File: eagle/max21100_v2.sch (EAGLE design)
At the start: 11 parts

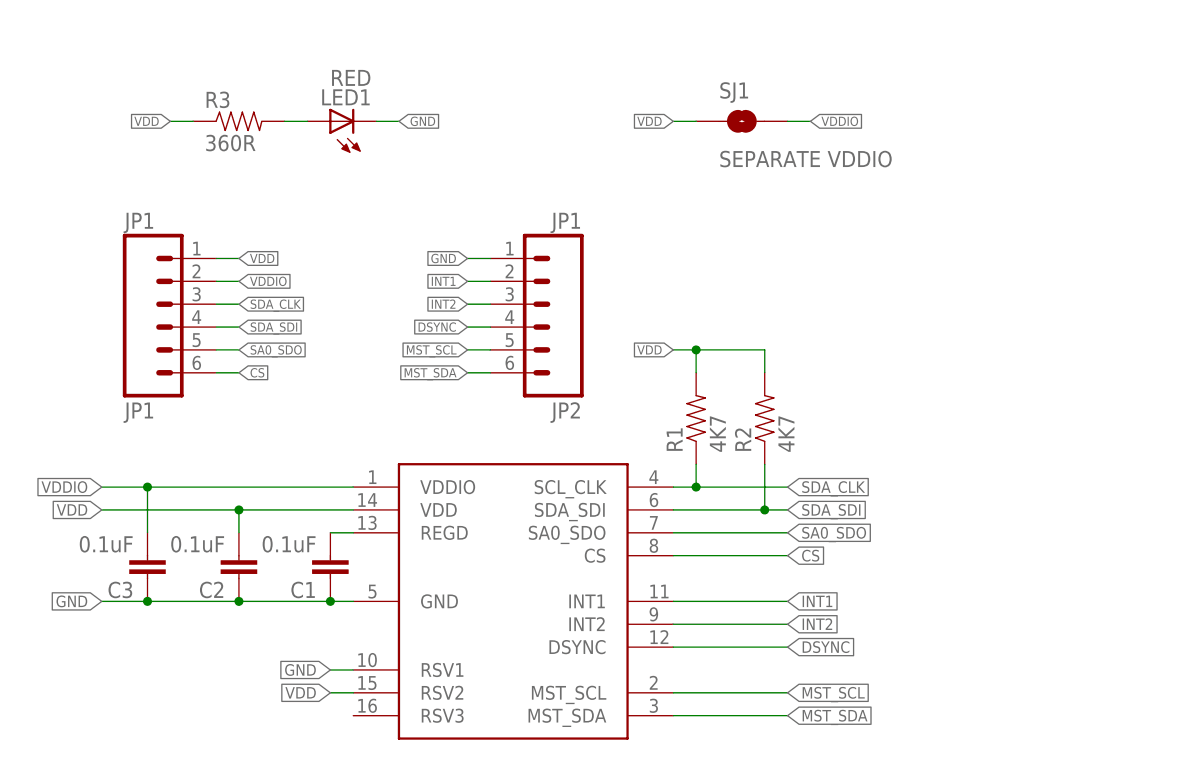
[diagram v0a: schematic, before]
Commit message: Improved V2
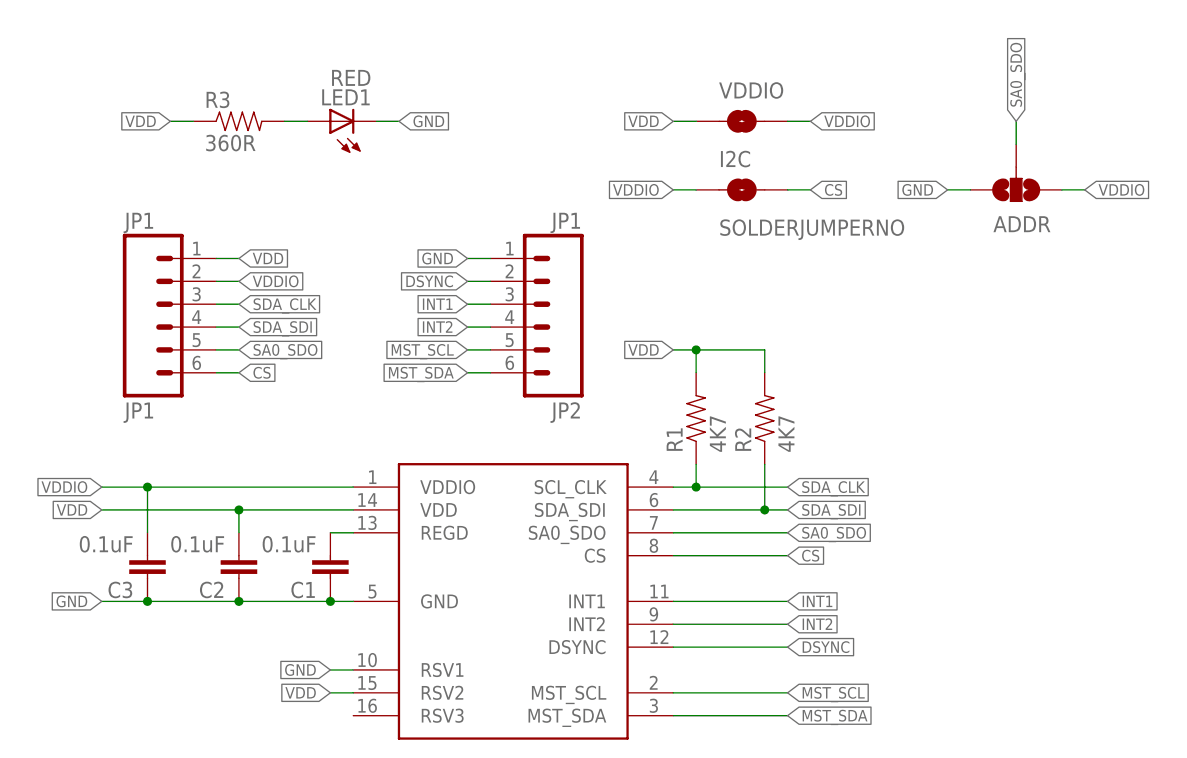
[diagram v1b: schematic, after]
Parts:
- added ADDR: (no value), max21100:SOLDERJUMPER_2WAYS
- added I2C: SOLDERJUMPERNO, max21100:SOLDERJUMPERNO
- VDDIO: value SEPARATE VDDIO -> SOLDERJUMPERTRACE
- renumbered SJ1 to VDDIO
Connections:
- net CS: now also I2C.2
- net DSYNC: now also JP2.2; no longer JP2.4
- net GND: now also ADDR.1
- net INT1: now also JP2.3; no longer JP2.2
- net INT2: now also JP2.4; no longer JP2.3
- net SA0_SDO: now also ADDR.2
- net VDDIO: now also ADDR.3, I2C.1
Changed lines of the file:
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@@
 <part name="R3" library="SparkFun-Passives" deviceset="RESISTOR" device="0603-RES" value="360R"/>
 <part name="LED1" library="breakouts" deviceset="LED" device="CHIP-LED0603" value="RED"/>
-<part name="SJ1" library="max21100" deviceset="SOLDERJUMPER" device="TRACE" value="SEPARATE VDDIO"/>
+<part name="VDDIO" library="max21100" deviceset="SOLDERJUMPER" device="TRACE" value=""/>
+<part name="I2C" library="max21100" deviceset="SOLDERJUMPER" device="NO" value="SOLDERJUMPERNO"/>
+<part name="ADDR" library="max21100" deviceset="SOLDERJUMPER_2WAY" device="S"/>
 </parts>
 <sheets>
@@
 <instance part="R3" gate="G$1" x="40.64" y="99.06"/>
 <instance part="LED1" gate="G$1" x="50.8" y="99.06" rot="R90"/>
-<instance part="SJ1" gate="1" x="96.52" y="99.06"/>
+<instance part="VDDIO" gate="1" x="96.52" y="99.06"/>
+<instance part="I2C" gate="1" x="96.52" y="91.44"/>
+<instance part="ADDR" gate="G$1" x="127" y="91.44" smashed="yes" rot="MR270">
+<attribute name="NAME" x="124.46" y="88.519" size="1.778" layer="95" rot="MR180"/>
+<attribute name="VALUE" x="128.905" y="88.9" size="1.778" layer="96" rot="MR270"/>
+</instance>
 </instances>
 <busses>
@@
 <segment>
 <wire x1="55.88" y1="99.06" x2="58.42" y2="99.06" width="0.1524" layer="91"/>
-<label x="58.42" y="99.06" size="1.016" layer="95" xref="yes"/>
+<label x="58.42" y="99.06" size="1.27" layer="95" xref="yes"/>
 <pinref part="LED1" gate="G$1" pin="C"/>
 </segment>
@@
 <pinref part="JP2" gate="G$1" pin="1"/>
 <wire x1="68.58" y1="83.82" x2="66.04" y2="83.82" width="0.1524" layer="91"/>
-<label x="66.04" y="83.82" size="1.016" layer="95" rot="R180" xref="yes"/>
+<label x="66.04" y="83.82" size="1.27" layer="95" rot="R180" xref="yes"/>
+</segment>
+<segment>
+<pinref part="ADDR" gate="G$1" pin="1"/>
+<wire x1="121.92" y1="91.44" x2="119.38" y2="91.44" width="0.1524" layer="91"/>
+<label x="119.38" y="91.44" size="1.27" layer="95" rot="R180" xref="yes"/>
 </segment>
 </net>
@@
 <wire x1="91.44" y1="73.66" x2="88.9" y2="73.66" width="0.1524" layer="91"/>
 <junction x="91.44" y="73.66"/>
-<label x="88.9" y="73.66" size="1.016" layer="95" rot="R180" xref="yes"/>
+<label x="88.9" y="73.66" size="1.27" layer="95" rot="R180" xref="yes"/>
 </segment>
 <segment>
 <wire x1="33.02" y1="99.06" x2="35.56" y2="99.06" width="0.1524" layer="91"/>
-<label x="33.02" y="99.06" size="1.016" layer="95" rot="R180" xref="yes"/>
+<label x="33.02" y="99.06" size="1.27" layer="95" rot="R180" xref="yes"/>
 <pinref part="R3" gate="G$1" pin="1"/>
 </segment>
@@
 <pinref part="JP1" gate="G$1" pin="1"/>
 <wire x1="38.1" y1="83.82" x2="40.64" y2="83.82" width="0.1524" layer="91"/>
-<label x="40.64" y="83.82" size="1.016" layer="95" xref="yes"/>
-</segment>
-<segment>
-<pinref part="SJ1" gate="1" pin="1"/>
+<label x="40.64" y="83.82" size="1.27" layer="95" xref="yes"/>
+</segment>
+<segment>
+<pinref part="VDDIO" gate="1" pin="1"/>
 <wire x1="91.44" y1="99.06" x2="88.9" y2="99.06" width="0.1524" layer="91"/>
-<label x="88.9" y="99.06" size="1.016" layer="95" rot="R180" xref="yes"/>
+<label x="88.9" y="99.06" size="1.27" layer="95" rot="R180" xref="yes"/>
 </segment>
 </net>
@@
 <pinref part="JP1" gate="G$1" pin="2"/>
 <wire x1="38.1" y1="81.28" x2="40.64" y2="81.28" width="0.1524" layer="91"/>
-<label x="40.64" y="81.28" size="1.016" layer="95" xref="yes"/>
-</segment>
-<segment>
-<pinref part="SJ1" gate="1" pin="2"/>
+<label x="40.64" y="81.28" size="1.27" layer="95" xref="yes"/>
+</segment>
+<segment>
+<pinref part="VDDIO" gate="1" pin="2"/>
 <wire x1="101.6" y1="99.06" x2="104.14" y2="99.06" width="0.1524" layer="91"/>
-<label x="104.14" y="99.06" size="1.016" layer="95" xref="yes"/>
+<label x="104.14" y="99.06" size="1.27" layer="95" xref="yes"/>
+</segment>
+<segment>
+<pinref part="I2C" gate="1" pin="1"/>
+<wire x1="91.44" y1="91.44" x2="88.9" y2="91.44" width="0.1524" layer="91"/>
+<label x="88.9" y="91.44" size="1.27" layer="95" rot="R180" xref="yes"/>
+</segment>
+<segment>
+<pinref part="ADDR" gate="G$1" pin="3"/>
+<wire x1="132.08" y1="91.44" x2="134.62" y2="91.44" width="0.1524" layer="91"/>
+<label x="134.62" y="91.44" size="1.27" layer="95" xref="yes"/>
 </segment>
 </net>
@@
 </segment>
 <segment>
-<pinref part="JP2" gate="G$1" pin="4"/>
-<wire x1="68.58" y1="76.2" x2="66.04" y2="76.2" width="0.1524" layer="91"/>
-<label x="66.04" y="76.2" size="1.016" layer="95" rot="R180" xref="yes"/>
+<pinref part="JP2" gate="G$1" pin="2"/>
+<wire x1="68.58" y1="81.28" x2="66.04" y2="81.28" width="0.1524" layer="91"/>
+<label x="66.04" y="81.28" size="1.27" layer="95" rot="R180" xref="yes"/>
 </segment>
 </net>
@@
 </segment>
 <segment>
-<pinref part="JP2" gate="G$1" pin="3"/>
-<wire x1="68.58" y1="78.74" x2="66.04" y2="78.74" width="0.1524" layer="91"/>
-<label x="66.04" y="78.74" size="1.016" layer="95" rot="R180" xref="yes"/>
+<pinref part="JP2" gate="G$1" pin="4"/>
+<wire x1="68.58" y1="76.2" x2="66.04" y2="76.2" width="0.1524" layer="91"/>
+<label x="66.04" y="76.2" size="1.27" layer="95" rot="R180" xref="yes"/>
 </segment>
 </net>
@@
 </segment>
 <segment>
-<pinref part="JP2" gate="G$1" pin="2"/>
-<wire x1="68.58" y1="81.28" x2="66.04" y2="81.28" width="0.1524" layer="91"/>
-<label x="66.04" y="81.28" size="1.016" layer="95" rot="R180" xref="yes"/>
+<pinref part="JP2" gate="G$1" pin="3"/>
+<wire x1="68.58" y1="78.74" x2="66.04" y2="78.74" width="0.1524" layer="91"/>
+<label x="66.04" y="78.74" size="1.27" layer="95" rot="R180" xref="yes"/>
 </segment>
 </net>
@@
 <pinref part="JP2" gate="G$1" pin="6"/>
 <wire x1="68.58" y1="71.12" x2="66.04" y2="71.12" width="0.1524" layer="91"/>
-<label x="66.04" y="71.12" size="1.016" layer="95" rot="R180" xref="yes"/>
+<label x="66.04" y="71.12" size="1.27" layer="95" rot="R180" xref="yes"/>
 </segment>
 </net>
@@
 <pinref part="JP2" gate="G$1" pin="5"/>
 <wire x1="68.58" y1="73.66" x2="66.04" y2="73.66" width="0.1524" layer="91"/>
-<label x="66.04" y="73.66" size="1.016" layer="95" rot="R180" xref="yes"/>
+<label x="66.04" y="73.66" size="1.27" layer="95" rot="R180" xref="yes"/>
 </segment>
 </net>
@@
 <pinref part="JP1" gate="G$1" pin="6"/>
 <wire x1="38.1" y1="71.12" x2="40.64" y2="71.12" width="0.1524" layer="91"/>
-<label x="40.64" y="71.12" size="1.016" layer="95" xref="yes"/>
+<label x="40.64" y="71.12" size="1.27" layer="95" xref="yes"/>
+</segment>
+<segment>
+<pinref part="I2C" gate="1" pin="2"/>
+<wire x1="101.6" y1="91.44" x2="104.14" y2="91.44" width="0.1524" layer="91"/>
+<label x="104.14" y="91.44" size="1.27" layer="95" xref="yes"/>
 </segment>
 </net>
@@
 <pinref part="JP1" gate="G$1" pin="5"/>
 <wire x1="38.1" y1="73.66" x2="40.64" y2="73.66" width="0.1524" layer="91"/>
-<label x="40.64" y="73.66" size="1.016" layer="95" xref="yes"/>
+<label x="40.64" y="73.66" size="1.27" layer="95" xref="yes"/>
+</segment>
+<segment>
+<pinref part="ADDR" gate="G$1" pin="2"/>
+<wire x1="127" y1="96.52" x2="127" y2="99.06" width="0.1524" layer="91"/>
+<label x="127" y="99.06" size="1.27" layer="95" rot="R90" xref="yes"/>
 </segment>
 </net>
@@
 <pinref part="JP1" gate="G$1" pin="4"/>
 <wire x1="38.1" y1="76.2" x2="40.64" y2="76.2" width="0.1524" layer="91"/>
-<label x="40.64" y="76.2" size="1.016" layer="95" xref="yes"/>
+<label x="40.64" y="76.2" size="1.27" layer="95" xref="yes"/>
 </segment>
 </net>
@@
 <pinref part="JP1" gate="G$1" pin="3"/>
 <wire x1="38.1" y1="78.74" x2="40.64" y2="78.74" width="0.1524" layer="91"/>
-<label x="40.64" y="78.74" size="1.016" layer="95" xref="yes"/>
-</segment>
-</net>
+<label x="40.64" y="78.74" size="1.27" layer="95" xref="yes"/>
+</segment>
+</net>
